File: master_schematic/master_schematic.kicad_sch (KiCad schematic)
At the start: 9 parts, among them Q1 IRLZ34NPBF, U1 teensy_4.1

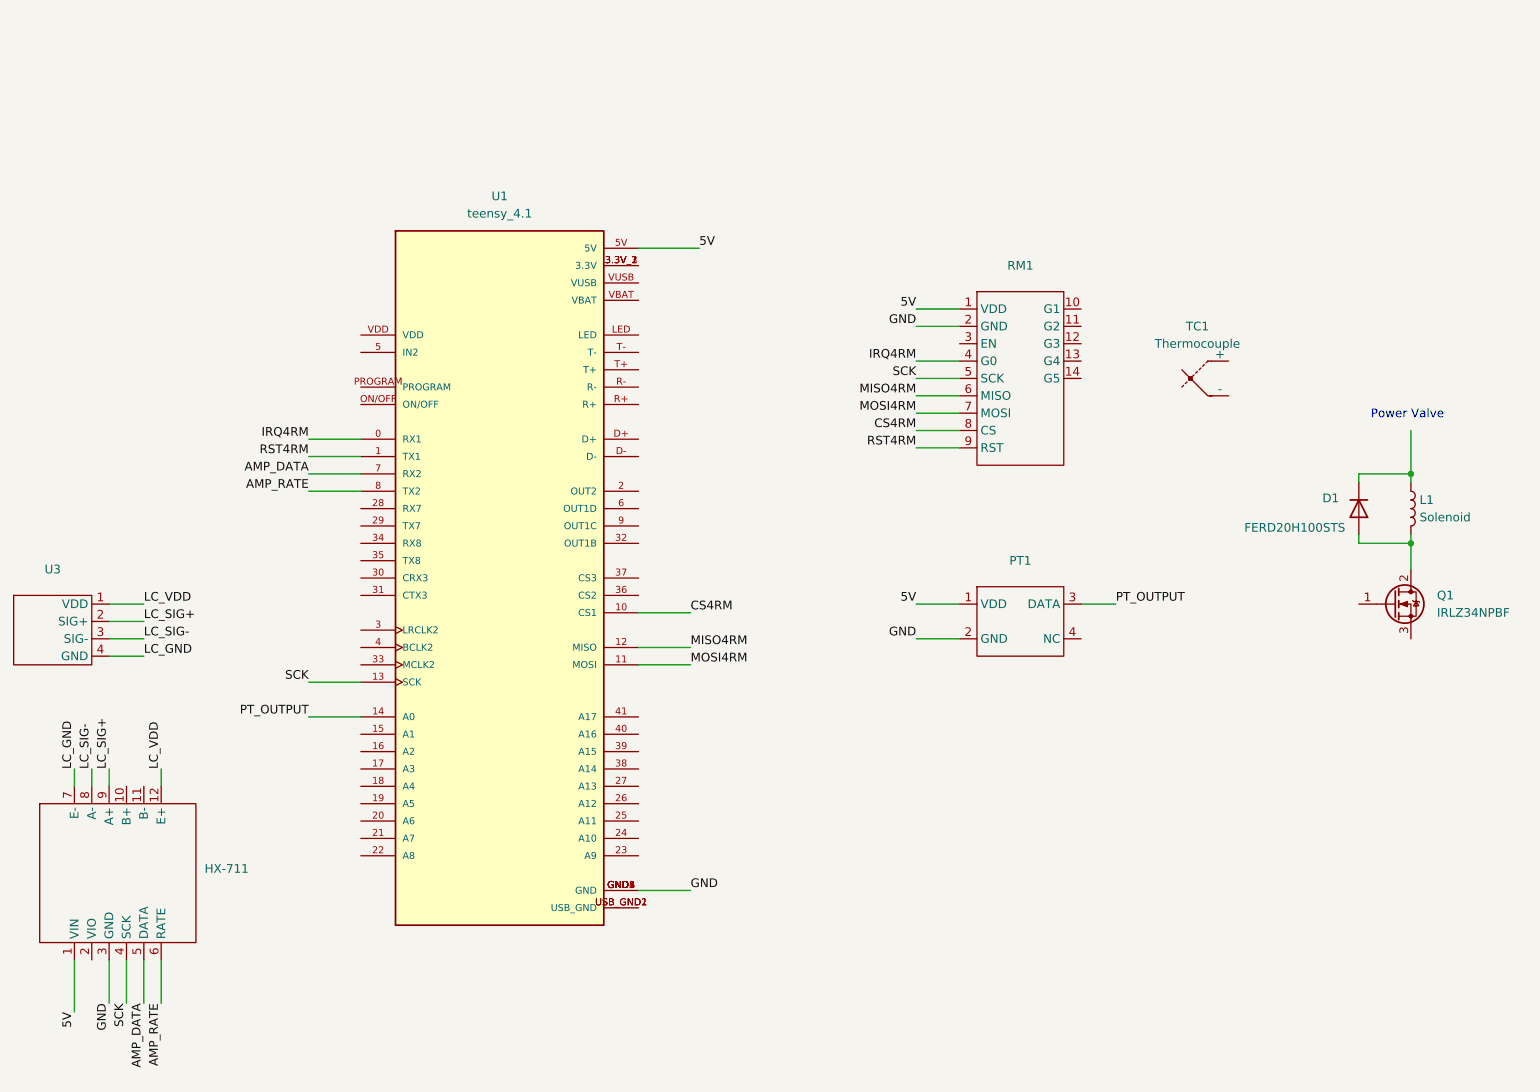
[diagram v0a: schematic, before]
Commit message: added sheet and connections for PT
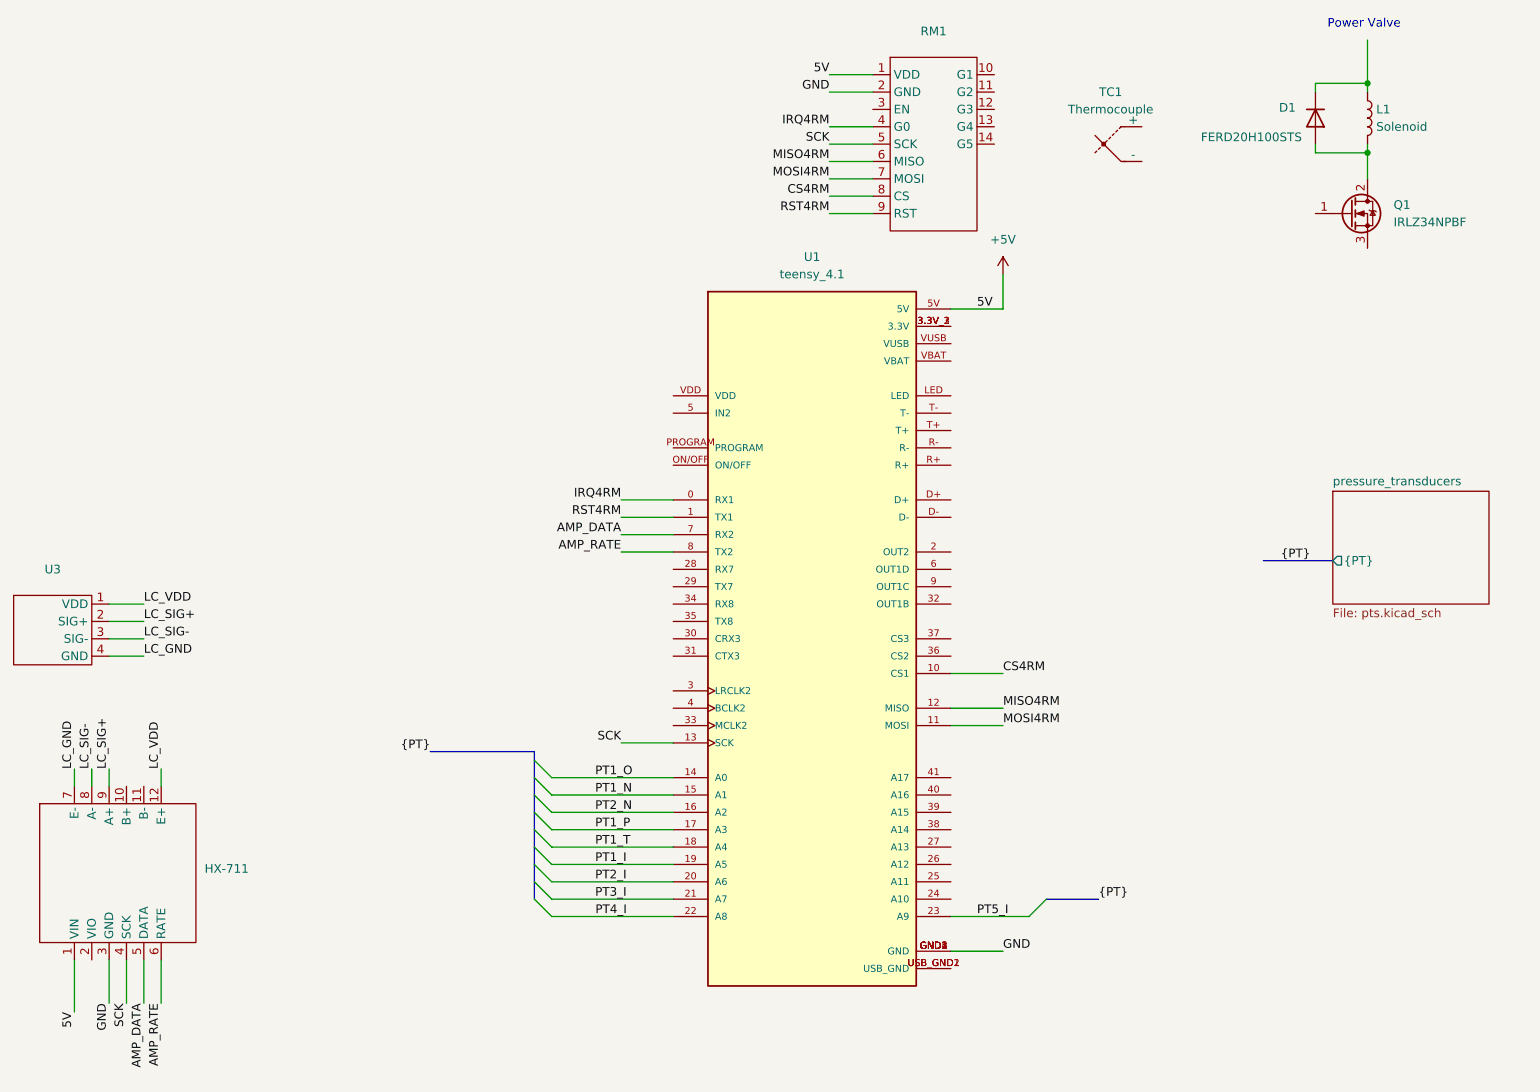
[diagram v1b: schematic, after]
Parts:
- removed PT1: ~, hb_footprint_lib:Pressure Transducer (Low), symbol hb_symbol_lib:pressure_transducer
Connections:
- net PT1_N: now reaches U1.15 (A1)
- net PT2_N: now reaches U1.16 (A2)
- net PT1_P: now reaches U1.17 (A3)
- net PT1_T: now reaches U1.18 (A4)
- net PT1_I: now reaches U1.19 (A5)
- net PT2_I: now reaches U1.20 (A6)
- net PT3_I: now reaches U1.21 (A7)
- net PT4_I: now reaches U1.22 (A8)
- net PT5_I: now reaches U1.23 (A9)
- net 5V renamed +5V
- net PT_OUTPUT renamed PT1_O
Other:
- added sheet pressure_transducers (pts.kicad_sch)
- moved on the sheet: D1, L1, Q1, RM1, TC1, U1
